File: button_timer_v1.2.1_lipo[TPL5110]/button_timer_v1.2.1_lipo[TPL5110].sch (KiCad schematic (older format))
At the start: 23 parts, among them J1 Conn_01x05_Female, SW1 SW_Push, SW2 SW_Push, U2 AP2112K-3.3, U3 TPL5111, X1 ESP-12E

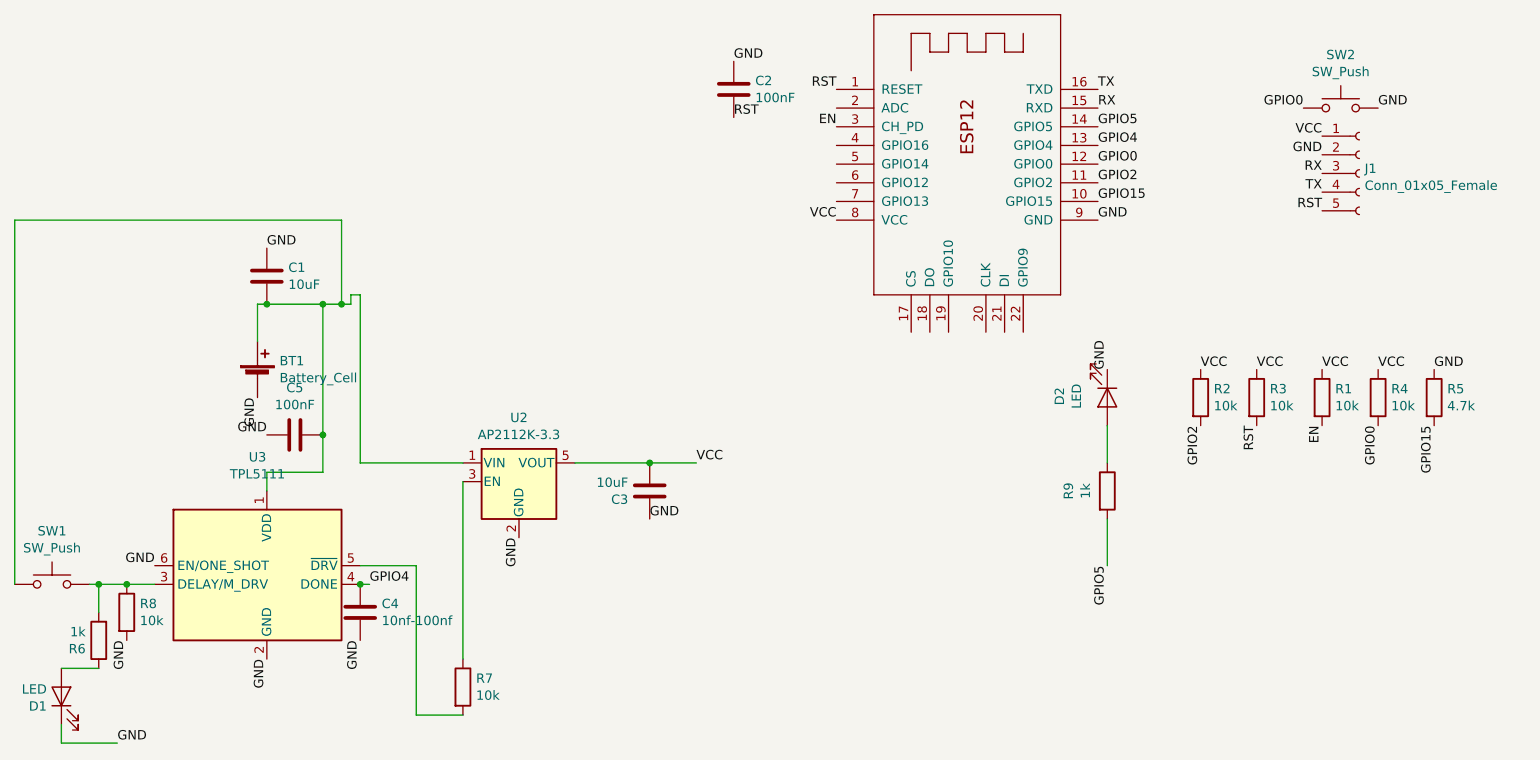
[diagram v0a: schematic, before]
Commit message: 23.02 13:31
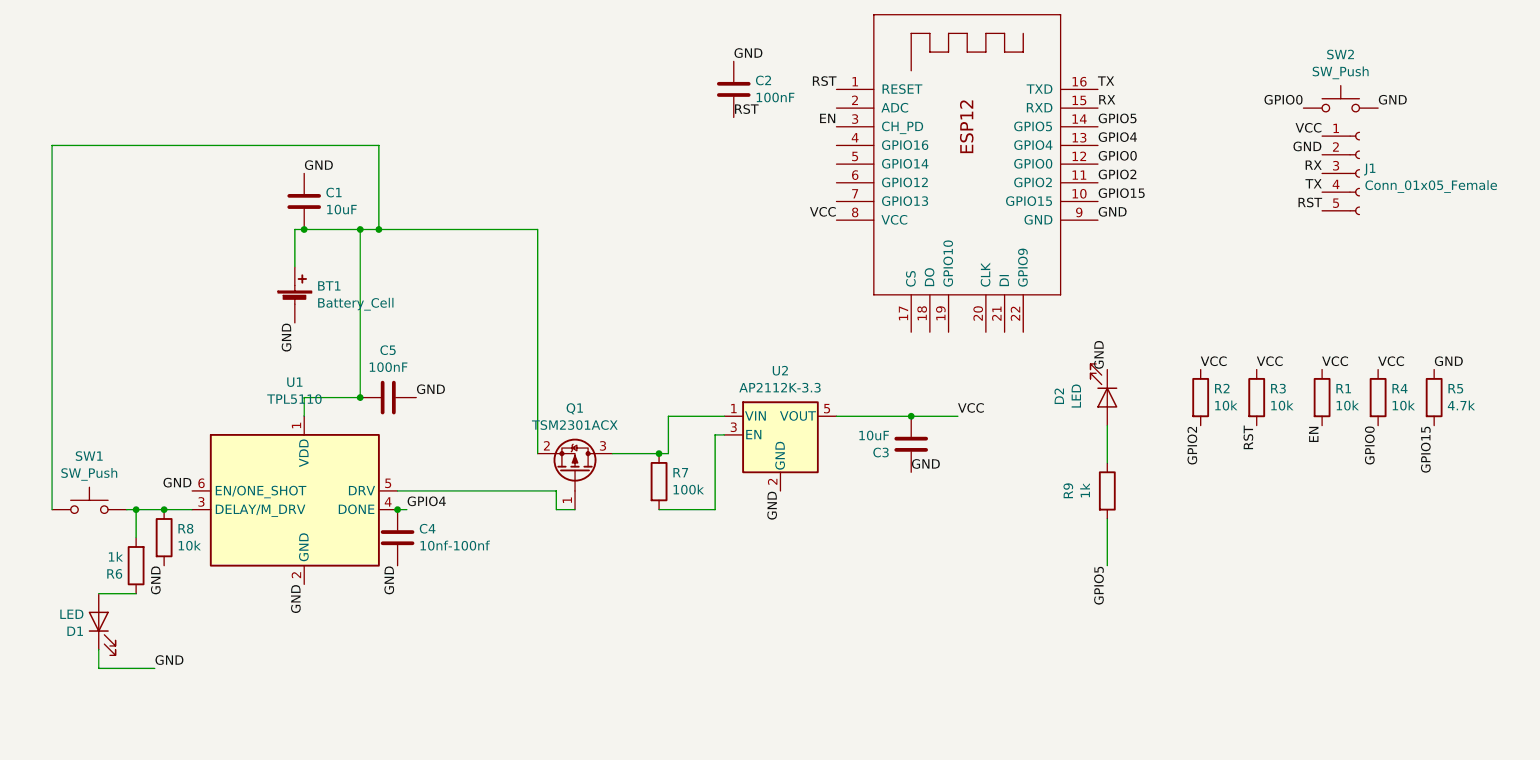
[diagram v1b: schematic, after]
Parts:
- removed R7: 10k, handsolder:R_0805_2012handsoldermod, symbol button-timer-v1.2-rescue:R-Device-button-timer-rescue-button-timer-v1.2-rescue-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
- removed U3: TPL5111, handsolder:SOT-23-6handsoldering, symbol button-timer-v1.2-rescue:TPL5111-Timer-button-timer-rescue-button-timer-v1.2-re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
- added Q1: TSM2301ACX, Package_TO_SOT_SMD:SOT-23, symbol Transistor_FET:TSM2301ACX
- added R7: 100k, handsolder:R_0805_2012handsoldermod, symbol Device:R
- added U1: TPL5110, handsolder:SOT-23-6handsoldering, symbol Timer:TPL5110
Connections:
- net GND: now also C5.1, U1.2 (GND), U1.6 (EN/ONE_SHOT); no longer C5.2
- net GPIO4: now also U1.4 (DONE)
- net at BT1.1 (+), C1.2, SW1.1: now also C5.2, Q1.2 (S), U1.1 (VDD); no longer C5.1, U2.1 (VIN)
- net at R6.2, R8.1, SW1.2: now also U1.3 (DELAY/M_DRV)
- net at U2.3 (EN): now also R7.2
- new net: Q1.3 (D), R7.1, U2.1 (VIN)
- new net: Q1.1 (G), U1.5 (DRV)
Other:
- moved on the sheet: BT1, C1, C3, C4, D1, R6, R8, SW1, U2

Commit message: 3D Models etwas verbessert
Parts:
- J1: footprint Connector_PinHeader_2.54mm:PinHeader_1x05_P2.54mm_Vertical -> handsolder:PinSocket_1x05_P2.54mm_Vertical_mod
- SW1: footprint Button_Switch_THT:SW_PUSH_6mm -> handsolder:SW_PUSH_6mm_H8mm_mod
- SW2: footprint Button_Switch_SMD:SW_SPST_EVQPE1 -> handsolder:SW_SPST_B3U-1000P_mod
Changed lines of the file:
@@
 F 0 "SW2" H 8000 3385 50  0000 C CNN
 F 1 "SW_Push" H 8000 3294 50  0000 C CNN
-F 2 "Button_Switch_SMD:SW_SPST_EVQPE1" H 8000 3300 50  0001 C CNN
+F 2 "handsolder:SW_SPST_B3U-1000P_mod" H 8000 3300 50  0001 C CNN
 F 3 "~" H 8000 3300 50  0001 C CNN
 	1    8000 3100
@@
 F 0 "SW1" H 1300 5535 50  0000 C CNN
 F 1 "SW_Push" H 1300 5444 50  0000 C CNN
-F 2 "Button_Switch_THT:SW_PUSH_6mm" H 1300 5450 50  0001 C CNN
+F 2 "handsolder:SW_PUSH_6mm_H8mm_mod" H 1300 5450 50  0001 C CNN
 F 3 "~" H 1300 5450 50  0001 C CNN
 	1    1300 5250
@@
 F 0 "J1" H 8128 3476 50  0000 L CNN
 F 1 "Conn_01x05_Female" H 8128 3385 50  0000 L CNN
-F 2 "Connector_PinHeader_2.54mm:PinHeader_1x05_P2.54mm_Vertical" H 8100 3450 50  0001 C CNN
+F 2 "handsolder:PinSocket_1x05_P2.54mm_Vertical_mod" H 8100 3450 50  0001 C CNN
 F 3 "~" H 8100 3450 50  0001 C CNN
 	1    8100 3450
